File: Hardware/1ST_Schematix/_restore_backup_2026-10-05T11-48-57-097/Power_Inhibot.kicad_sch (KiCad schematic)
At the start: 50 parts, among them J301 USB_C_Receptacle_USB2.0_16P, J302 Conn_01x02, Q301 MMDT2222A, Q302 DMP1045U-7, Q303 DMN313DLT-7, U301 USBLC6-2SC6, U302 BQ25896RTW, U303 BQ27220YZFR, U305 BU33SD5WG-TR

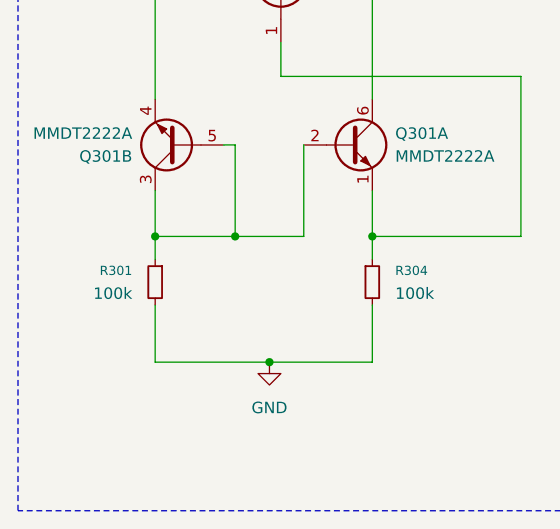
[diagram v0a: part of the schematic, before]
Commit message: midway
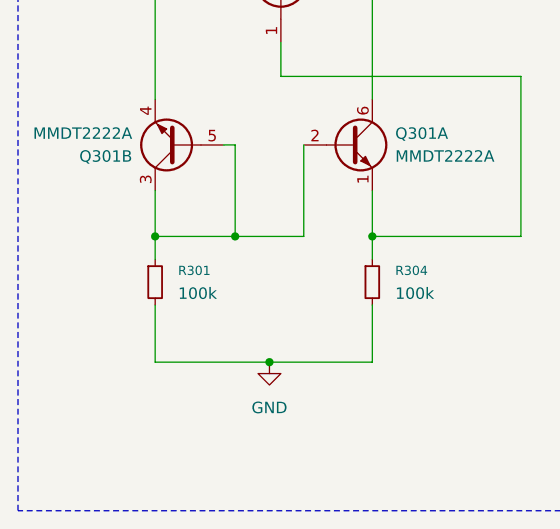
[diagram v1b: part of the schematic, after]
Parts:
- L301: footprint Inductor_SMD:L_0603_1608Metric -> Package_SO:SOIC-16_3.9x9.9mm_P1.27mm; JLCPCB Part # MPL1608S1R0MHT -> (none)
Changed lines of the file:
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@@
 			)
 		)
-		(property "Footprint" "Inductor_SMD:L_0603_1608Metric"
+		(property "Footprint" "Package_SO:SOIC-16_3.9x9.9mm_P1.27mm"
 			(at 166.37 91.44 0)
 			(hide yes)
@@
 			)
 		)
-		(property "JLCPCB Part #" "MPL1608S1R0MHT"
-			(at 166.37 91.44 90)
-			(hide yes)
-			(show_name no)
-			(do_not_autoplace no)
-			(effects
-				(font
-					(size 1.27 1.27)
-				)
-			)
-		)
 		(pin "2"
 		)
@@
 		(lib_id "Device:R_Small")
 		(at 26.67 168.91 0)
-		(mirror y)
 		(unit 1)
 		(body_style 1)
@@
 		(in_pos_files yes)
 		(dnp no)
+		(fields_autoplaced yes)
 		(property "Reference" "R301"
-			(at 24.13 167.6399 0)
+			(at 29.21 167.6399 0)
 			(show_name no)
 			(do_not_autoplace no)
@@
 		)
 		(property "Value" "100k"
-			(at 24.13 170.1799 0)
+			(at 29.21 170.1799 0)
 			(show_name no)
 			(do_not_autoplace no)
